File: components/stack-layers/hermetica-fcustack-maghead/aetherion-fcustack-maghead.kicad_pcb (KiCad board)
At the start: 2 copper layers, 16 x 16 mm, 13 parts, among them IC1 STM-IIS2MDC, J1 Conn_01x01, J2 Conn_01x01, J3 Conn_01x01, J4 Conn_01x01, J5 Conn_01x01

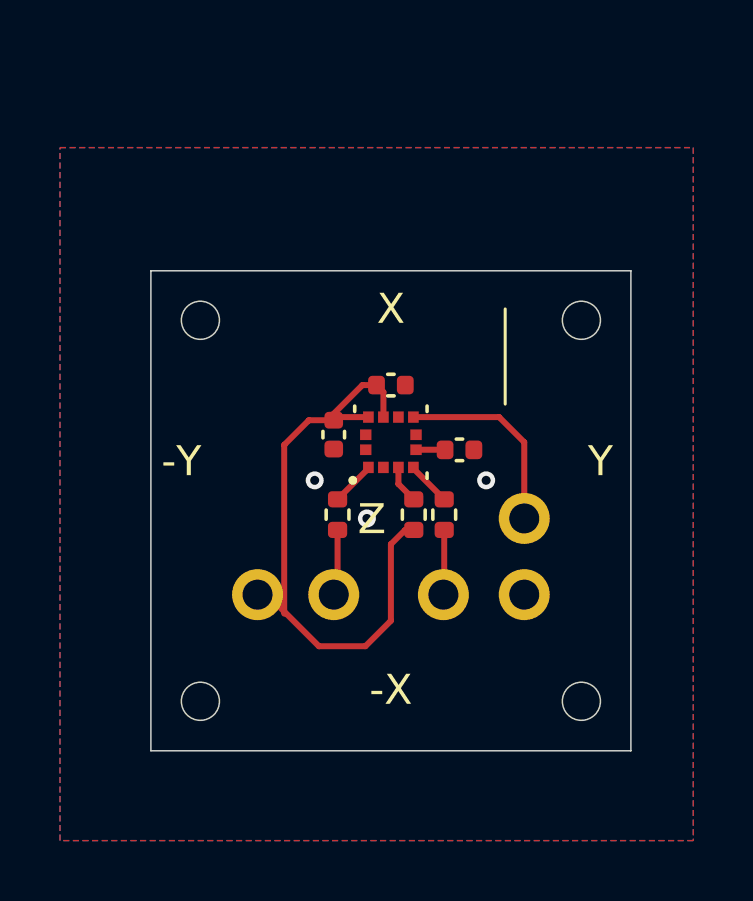
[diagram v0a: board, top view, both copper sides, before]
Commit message: updated pcbs
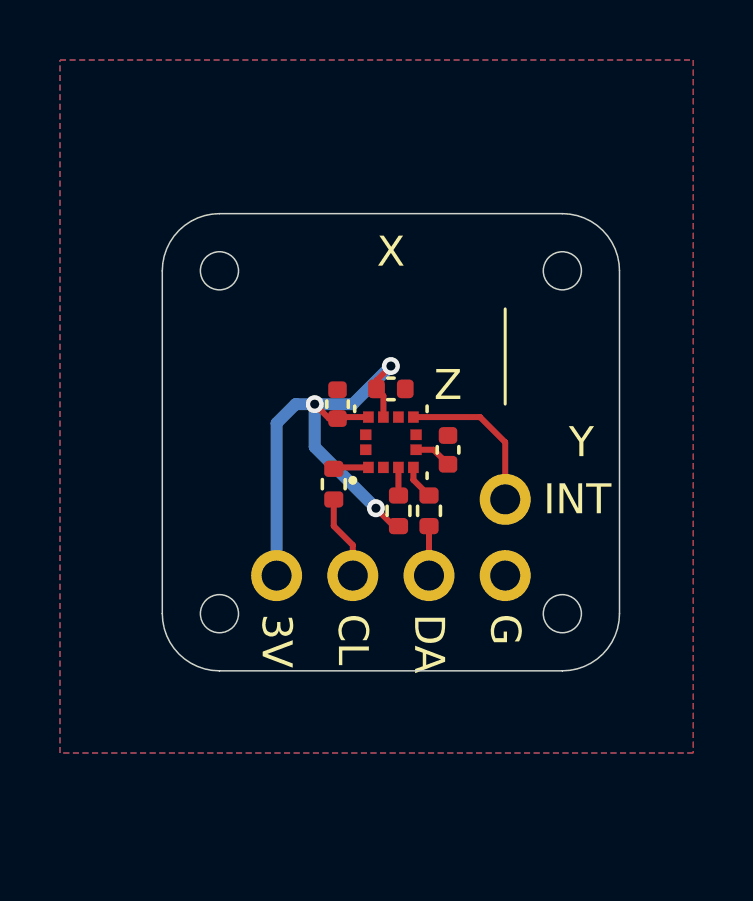
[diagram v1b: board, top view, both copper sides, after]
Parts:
- removed REF**: LOGO-HERMETICA, djStandard:LOGO-HERMETICA
- moved C2 1.02 mm to (-1.78, -1.27), turned to 90 degrees
- moved R1 1.02 mm to (-1.91, 1.40)
- moved J5 0.90 mm to (3.81, 1.91)
- moved J1 0.90 mm to (-3.81, 4.45)
- moved J2 0.90 mm to (3.81, 4.45)
- moved J3 0.90 mm to (-1.27, 4.45)
- moved J4 0.80 mm to (1.27, 4.45)
- moved R2 0.52 mm to (1.27, 2.29)
- moved R3 0.52 mm to (0.25, 2.29)
- moved C1 0.38 mm to (1.91, 0.25), turned to 90 degrees
- moved C3 0.13 mm to (0.00, -1.78)
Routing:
- net +VCC: track 20.5 -> 19.0 mm, vias 0 -> 3
- net /INT: track 6.58 -> 5.31 mm
- net /SCL: track 2.21 -> 3.06 mm
- net GND: vias 3 -> 0
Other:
- board size 16 x 16 mm -> 15.2 x 15.2 mm
- board text added: "-Z"
- board text added: "3V"
- board text added: "CL"
- board text added: "DA"
- board text added: "G"
- board text added: "INT"
- board text removed: "-X"
- board text removed: "-Y"
